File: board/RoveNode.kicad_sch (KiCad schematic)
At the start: 24 parts, among them J1 Conn_01x05, J3 Conn_01x24_Pin, J4 Conn_01x24_Pin, SW1 RST_Push, SW2 BOOT_Push, U1 STM32H563RITx, U3 SN65HVD232

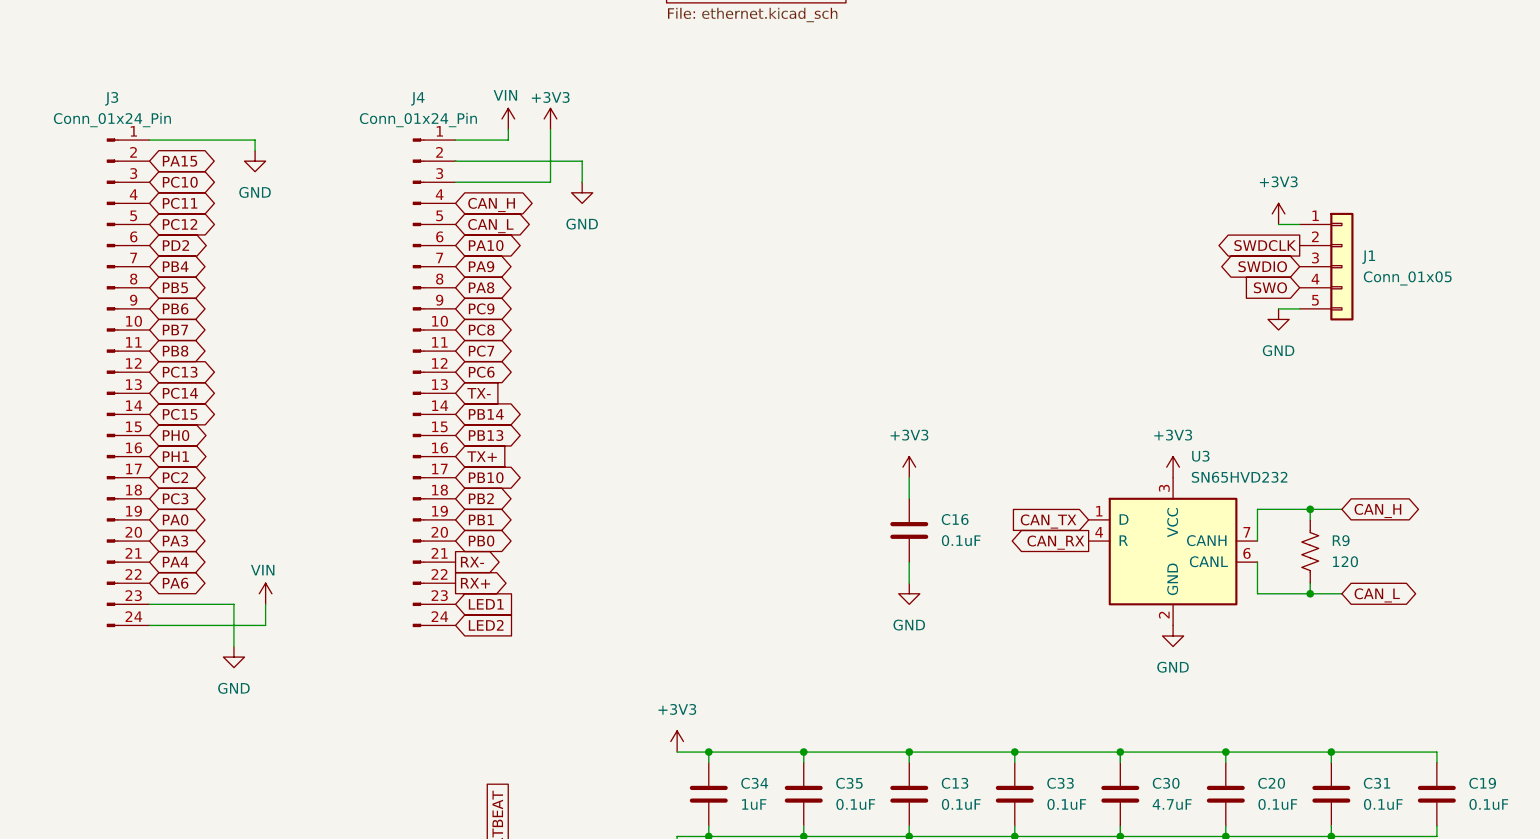
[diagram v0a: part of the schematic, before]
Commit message: Layout Complete
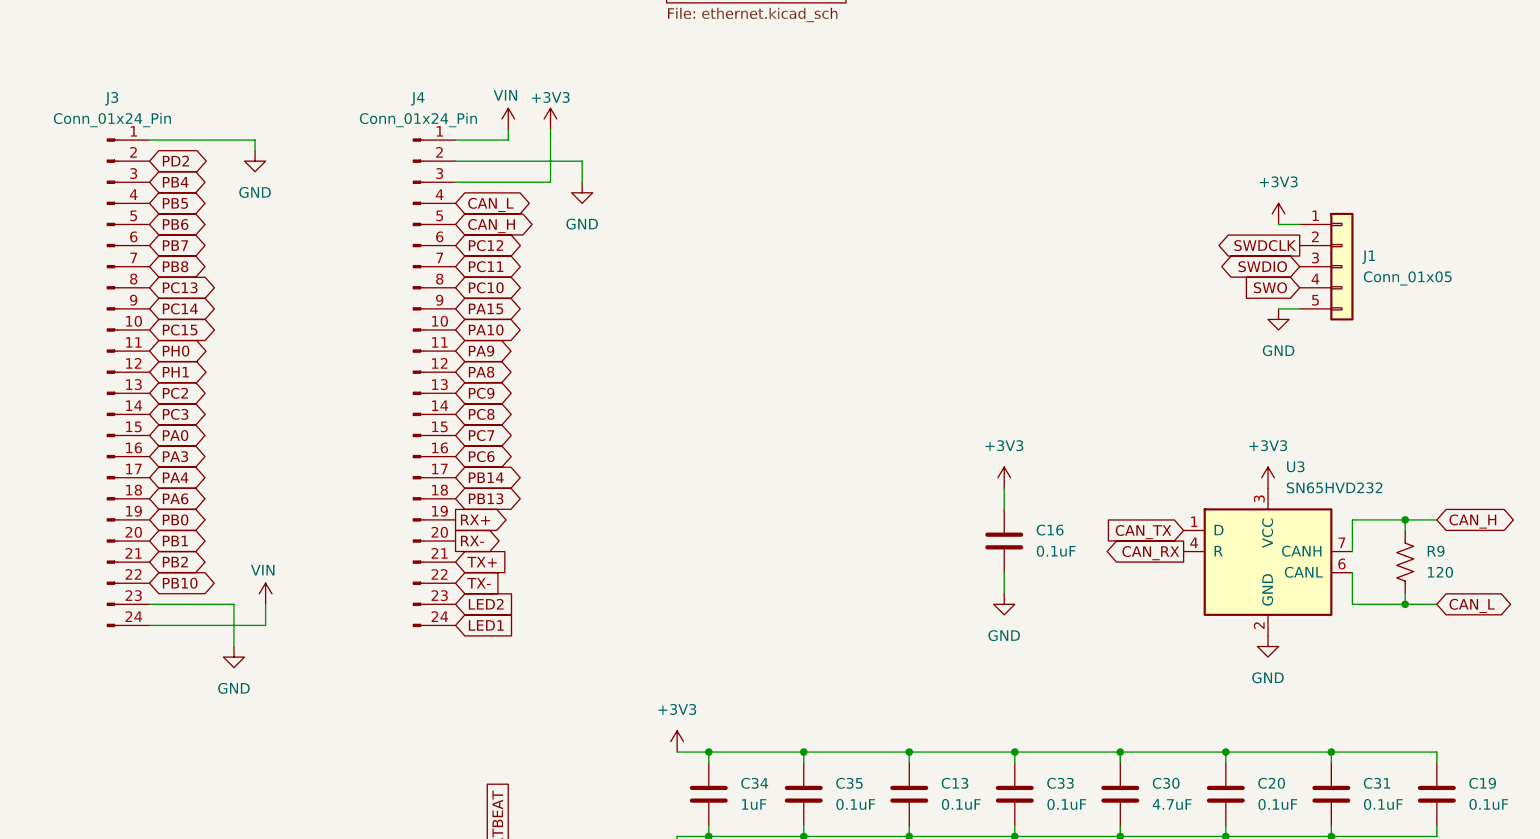
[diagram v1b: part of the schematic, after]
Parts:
- J1: footprint Connector_PinSocket_2.54mm:PinSocket_1x05_P2.54mm_Vertical -> Connector_JST:JST_PH_S5B-PH-K_1x05_P2.00mm_Horizontal
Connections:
- net CAN_H: now also J4.5 (Pin_5); no longer J4.4 (Pin_4)
- net CAN_L: now also J4.4 (Pin_4); no longer J4.5 (Pin_5)
- net LED1: now also J4.24 (Pin_24); no longer J4.23 (Pin_23)
- net LED2: now also J4.23 (Pin_23); no longer J4.24 (Pin_24)
- net PA0: now also J3.15 (Pin_15); no longer J3.19 (Pin_19)
- net PA10: now also J4.10 (Pin_10); no longer J4.6 (Pin_6)
- net PA15: now also J4.9 (Pin_9); no longer J3.2 (Pin_2)
- net PA3: now also J3.16 (Pin_16); no longer J3.20 (Pin_20)
- net PA4: now also J3.17 (Pin_17); no longer J3.21 (Pin_21)
- net PA6: now also J3.18 (Pin_18); no longer J3.22 (Pin_22)
- net PA8: now also J4.12 (Pin_12); no longer J4.8 (Pin_8)
- net PA9: now also J4.11 (Pin_11); no longer J4.7 (Pin_7)
- net PB0: now also J3.19 (Pin_19); no longer J4.20 (Pin_20)
- net PB1: now also J3.20 (Pin_20); no longer J4.19 (Pin_19)
- net PB10: now also J3.22 (Pin_22); no longer J4.17 (Pin_17)
- net PB13: now also J4.18 (Pin_18); no longer J4.15 (Pin_15)
- net PB14: now also J4.17 (Pin_17); no longer J4.14 (Pin_14)
- net PB2: now also J3.21 (Pin_21); no longer J4.18 (Pin_18)
- net PB4: now also J3.3 (Pin_3); no longer J3.7 (Pin_7)
- net PB5: now also J3.4 (Pin_4); no longer J3.8 (Pin_8)
- net PB6: now also J3.5 (Pin_5); no longer J3.9 (Pin_9)
- net PB7: now also J3.6 (Pin_6); no longer J3.10 (Pin_10)
- net PB8: now also J3.7 (Pin_7); no longer J3.11 (Pin_11)
- net PC10: now also J4.8 (Pin_8); no longer J3.3 (Pin_3)
- net PC11: now also J4.7 (Pin_7); no longer J3.4 (Pin_4)
- net PC12: now also J4.6 (Pin_6); no longer J3.5 (Pin_5)
- net PC13: now also J3.8 (Pin_8); no longer J3.12 (Pin_12)
- net PC14: now also J3.9 (Pin_9); no longer J3.13 (Pin_13)
- net PC15: now also J3.10 (Pin_10); no longer J3.14 (Pin_14)
- net PC2: now also J3.13 (Pin_13); no longer J3.17 (Pin_17)
- net PC3: now also J3.14 (Pin_14); no longer J3.18 (Pin_18)
- net PC6: now also J4.16 (Pin_16); no longer J4.12 (Pin_12)
- net PC7: now also J4.15 (Pin_15); no longer J4.11 (Pin_11)
- net PC8: now also J4.14 (Pin_14); no longer J4.10 (Pin_10)
- net PC9: now also J4.13 (Pin_13); no longer J4.9 (Pin_9)
- net PD2: now also J3.2 (Pin_2); no longer J3.6 (Pin_6)
- net PH0: now also J3.11 (Pin_11); no longer J3.15 (Pin_15)
- net PH1: now also J3.12 (Pin_12); no longer J3.16 (Pin_16)
- net RX+: now also J4.19 (Pin_19); no longer J4.22 (Pin_22)
- net RX-: now also J4.20 (Pin_20); no longer J4.21 (Pin_21)
- net TX+: now also J4.21 (Pin_21); no longer J4.16 (Pin_16)
- net TX-: now also J4.22 (Pin_22); no longer J4.13 (Pin_13)
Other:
- moved on the sheet: C16, R9, U3
